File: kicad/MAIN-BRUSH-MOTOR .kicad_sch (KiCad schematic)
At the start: 6 parts, among them J11 MAIN BRUSH, Q10 AO3400

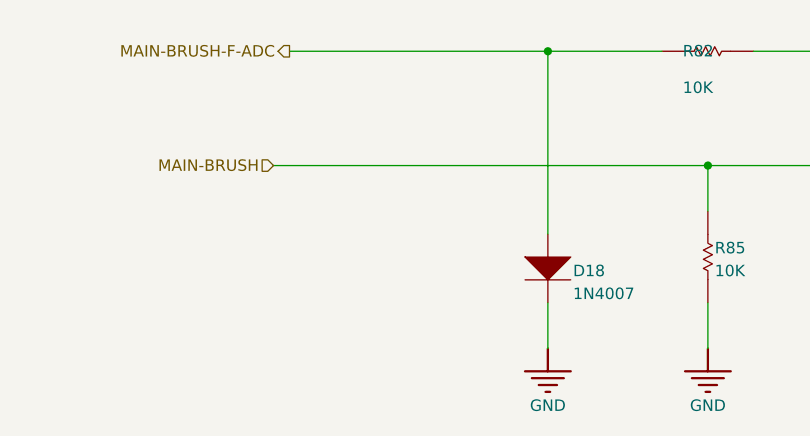
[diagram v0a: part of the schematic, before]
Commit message: Battery charging
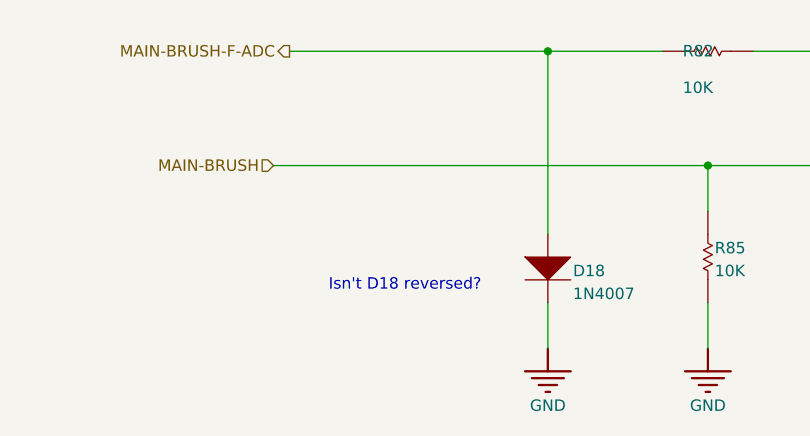
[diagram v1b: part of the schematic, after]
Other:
- note added: "Isn't D18 reversed?"
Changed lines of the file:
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@@
+		)
+	)
+	(text "Isn't D18 reversed?"
+		(exclude_from_sim no)
+		(at 234.315 217.805 0)
+		(effects
+			(font
+				(size 1.27 1.27)
+			)
 		)
 	)
